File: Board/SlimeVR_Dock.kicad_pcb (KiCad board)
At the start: 2 copper layers, 100 x 78 mm, 136 parts, among them J1Fan1 Conn_01x04_Pin, J1Temp1 Conn_01x05_Pin, J1_Control1 Conn_01x03_Pin, J1_MainPW1 USB_C_Receptacle_USB2.0_16P, J1_Monitor1 Conn_01x03_Pin, J1_Prog1 Conn_01x03_Pin, J2 USB_C_Receptacle_USB2.0_16P, J3 USB_C_Receptacle_USB2.0_16P, J4 USB_C_Receptacle_USB2.0_16P, J5 USB_C_Receptacle_USB2.0_16P, J6 USB_C_Receptacle_USB2.0_16P, J7 USB_C_Receptacle_USB2.0_16P, J8 USB_C_Receptacle_USB2.0_16P, J9 USB_C_Receptacle_USB2.0_16P, Q1 NDT452AP, Q2 BC857, Q3 BC857, Q4 BC857, Q5 BC857, Q6 BC817, U1 ESP32-C3-WROOM-02, U10 INA226, U11 AP22652W6-7, U12 INA226, U13 INA226, U14 AP22652W6-7, U15 INA226, U16 INA226, U17 74HC165, U18 74HC165, U19 74HC595, U2 CH224K, U3 XC6220B331MR, U4 TPS548A20RVER, U5 AP22652W6-7, U6 INA226, U7 INA226, U8 AP22652W6-7, U9 INA226

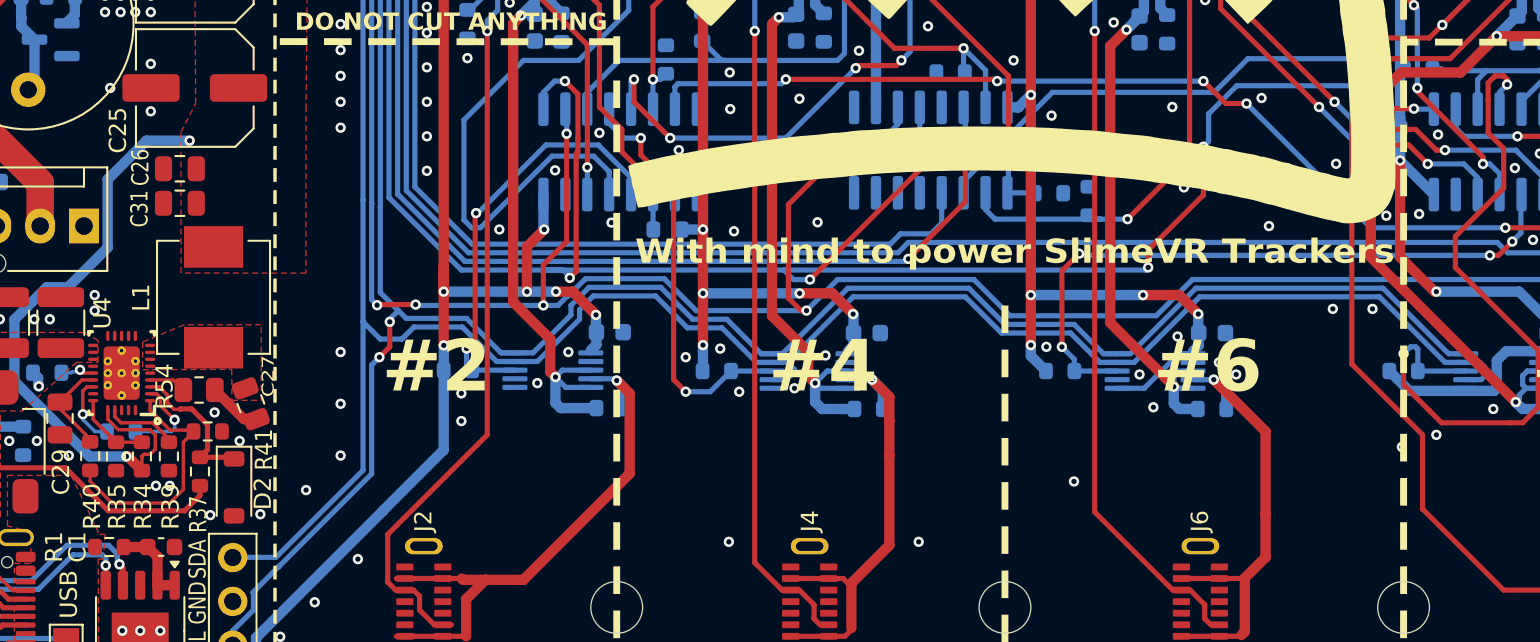
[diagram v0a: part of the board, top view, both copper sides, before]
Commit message: Changed baed on sugestions
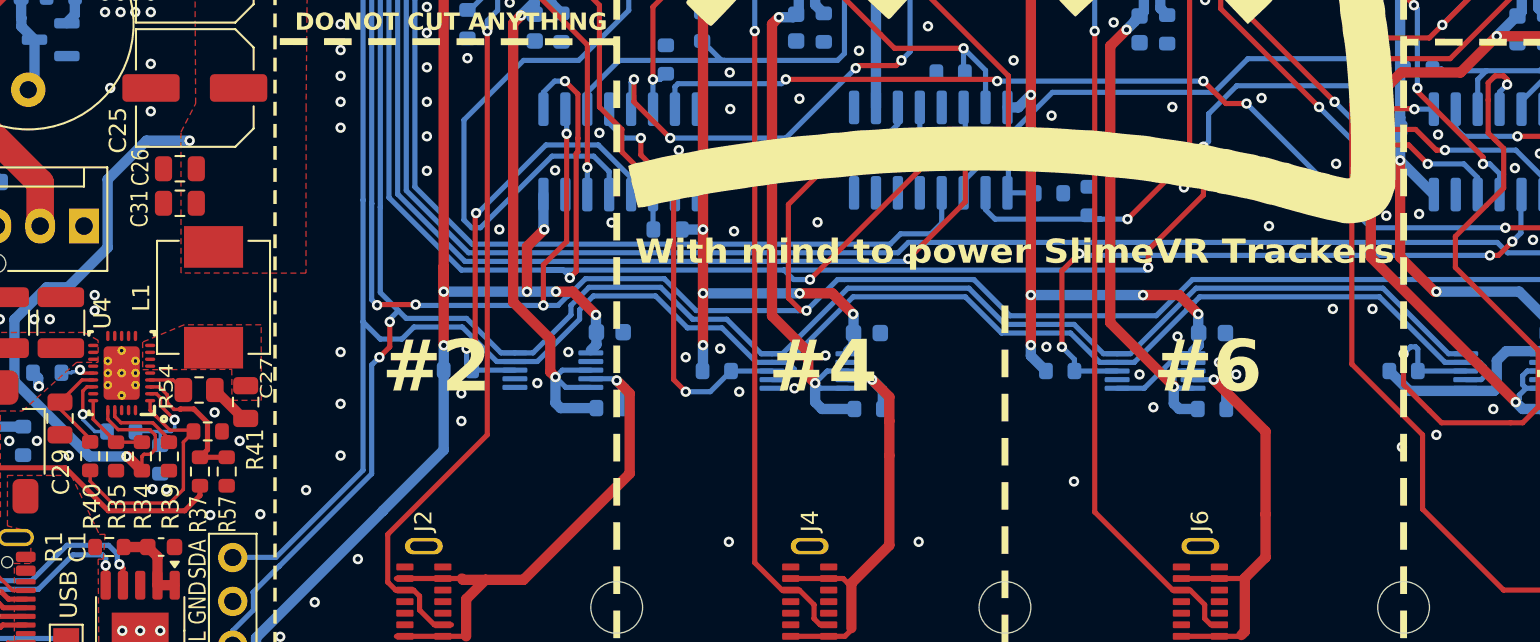
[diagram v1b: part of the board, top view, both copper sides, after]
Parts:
- removed D2: 5.1V, Diode_SMD:D_SOD-123
- added R56: 100k, Resistor_SMD:R_0603_1608Metric, B.Cu at (110.0, 122.7)
- added R57: 10k, Resistor_SMD:R_0603_1608Metric, F.Cu at (113.9, 123.4)
- R37: value 4k7 -> 75k
- moved C27 0.32 mm to (115.0, 119.4), turned to 90 degrees
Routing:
- net Net-(C27-Pad1): track 3.26 -> 2.46 mm
- net Net-(U4-PGOOD): track 5.15 -> 5.94 mm
